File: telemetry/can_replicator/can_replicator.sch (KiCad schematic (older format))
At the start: 31 parts, among them J1 CONN_02X03, U1 MCP2561-E_SN, U2 ATMEGA16M1, U3 USB_MicroB, U4 FT232RL, Y1 Crystal_SMD

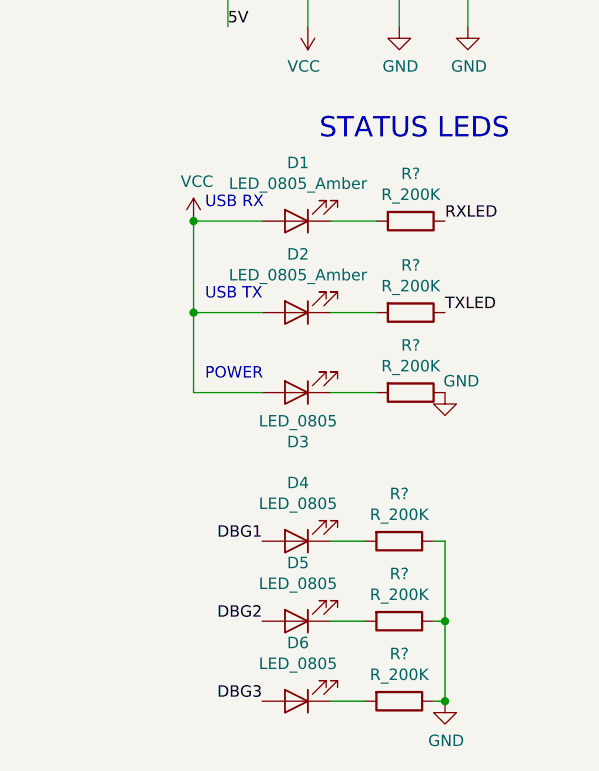
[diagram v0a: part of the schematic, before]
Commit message: chore: annotate schematic
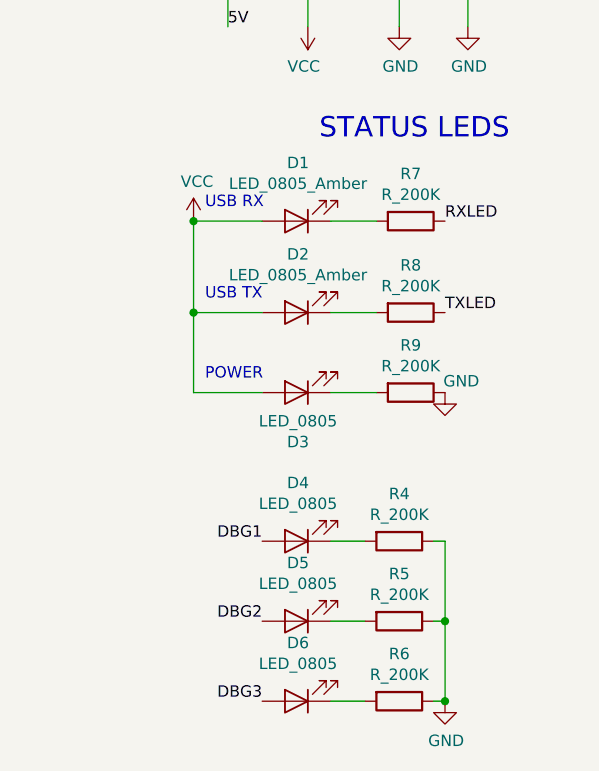
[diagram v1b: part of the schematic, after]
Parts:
- gave numbers to parts that had none: 6
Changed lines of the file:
@@
 $EndComp
 $Comp
-L power:GND #PWR?
+L power:GND #PWR024
 U 1 1 5FB7CF68
 P 15900 8850
-F 0 "#PWR?" H 15900 8600 50  0001 C CNN
+F 0 "#PWR024" H 15900 8600 50  0001 C CNN
 F 1 "GND" H 15905 8677 50  0000 C CNN
 F 2 "" H 15900 8850 50  0001 C CNN
@@
 NoConn ~ 3800 1600
 $Comp
-L formula:R_200K R?
+L formula:R_200K R7
 U 1 1 5FB83E8C
 P 15750 6750
-F 0 "R?" V 15543 6750 50  0000 C CNN
+F 0 "R7" V 15543 6750 50  0000 C CNN
 F 1 "R_200K" V 15634 6750 50  0000 C CNN
 F 2 "footprints:R_0805_OEM" H 15680 6750 50  0001 C CNN
@@
 $EndComp
 $Comp
-L formula:R_200K R?
+L formula:R_200K R8
 U 1 1 5FB8465B
 P 15750 7150
-F 0 "R?" V 15543 7150 50  0000 C CNN
+F 0 "R8" V 15543 7150 50  0000 C CNN
 F 1 "R_200K" V 15634 7150 50  0000 C CNN
 F 2 "footprints:R_0805_OEM" H 15680 7150 50  0001 C CNN
@@
 $EndComp
 $Comp
-L formula:R_200K R?
+L formula:R_200K R9
 U 1 1 5FB84F88
 P 15750 7500
-F 0 "R?" V 15543 7500 50  0000 C CNN
+F 0 "R9" V 15543 7500 50  0000 C CNN
 F 1 "R_200K" V 15634 7500 50  0000 C CNN
 F 2 "footprints:R_0805_OEM" H 15680 7500 50  0001 C CNN
@@
 $EndComp
 $Comp
-L formula:R_200K R?
+L formula:R_200K R4
 U 1 1 5FB85882
 P 15700 8150
-F 0 "R?" V 15493 8150 50  0000 C CNN
+F 0 "R4" V 15493 8150 50  0000 C CNN
 F 1 "R_200K" V 15584 8150 50  0000 C CNN
 F 2 "footprints:R_0805_OEM" H 15630 8150 50  0001 C CNN
@@
 	15850 8150 15900 8150
 $Comp
-L formula:R_200K R?
+L formula:R_200K R5
 U 1 1 5FB865BA
 P 15700 8500
-F 0 "R?" V 15493 8500 50  0000 C CNN
+F 0 "R5" V 15493 8500 50  0000 C CNN
 F 1 "R_200K" V 15584 8500 50  0000 C CNN
 F 2 "footprints:R_0805_OEM" H 15630 8500 50  0001 C CNN
@@
 	15850 8500 15900 8500
 $Comp
-L formula:R_200K R?
+L formula:R_200K R6
 U 1 1 5FB86F49
 P 15700 8850
-F 0 "R?" V 15493 8850 50  0000 C CNN
+F 0 "R6" V 15493 8850 50  0000 C CNN
 F 1 "R_200K" V 15584 8850 50  0000 C CNN
 F 2 "footprints:R_0805_OEM" H 15630 8850 50  0001 C CNN
